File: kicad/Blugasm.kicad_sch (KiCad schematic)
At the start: 46 parts, among them J1 PWR, J2 OLED, J3 I2C, J4 SERVO1, J5 PJ-102AH, J6 SERVO2, J7 BATT, Q1 DMG3415U, Q2 Q_NMOS_DGS, SW1 PWR, SW2 PEC11R-4225F-50024, U1 MCP73831-2-OT, U2 MP3V5050GP, U3 MCP6001-OT, U4 AP2112K-3.3

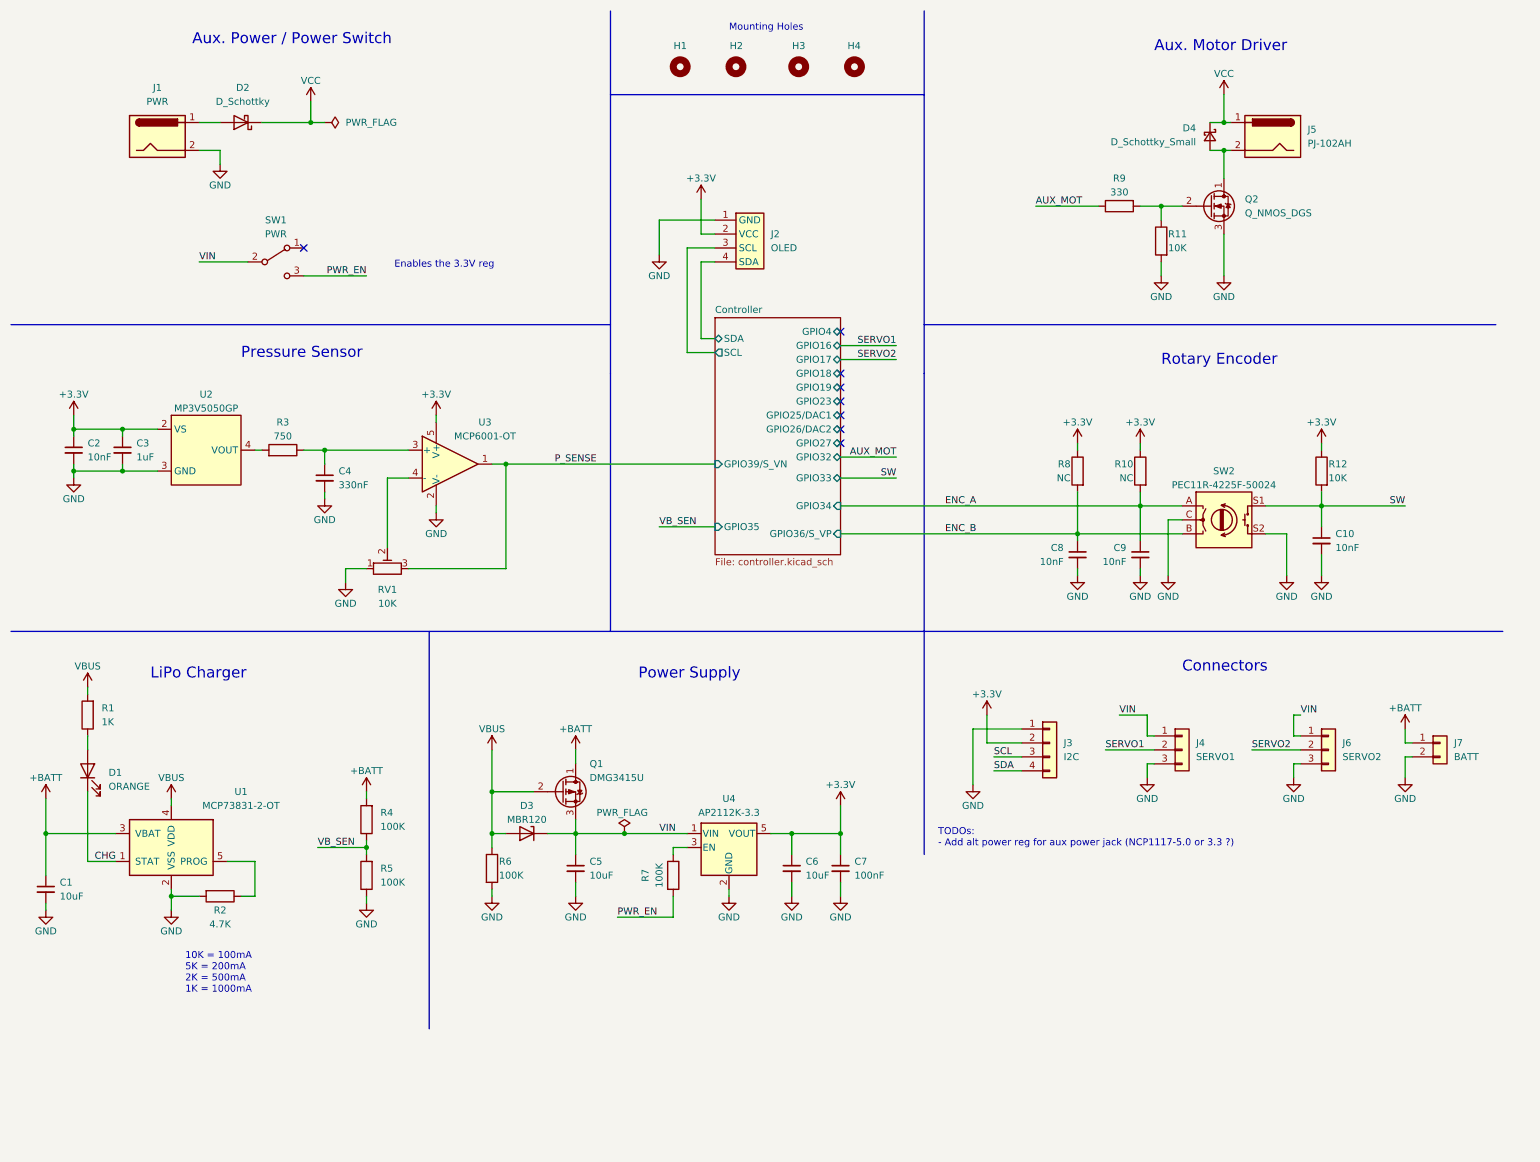
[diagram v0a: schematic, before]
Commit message: cleanup
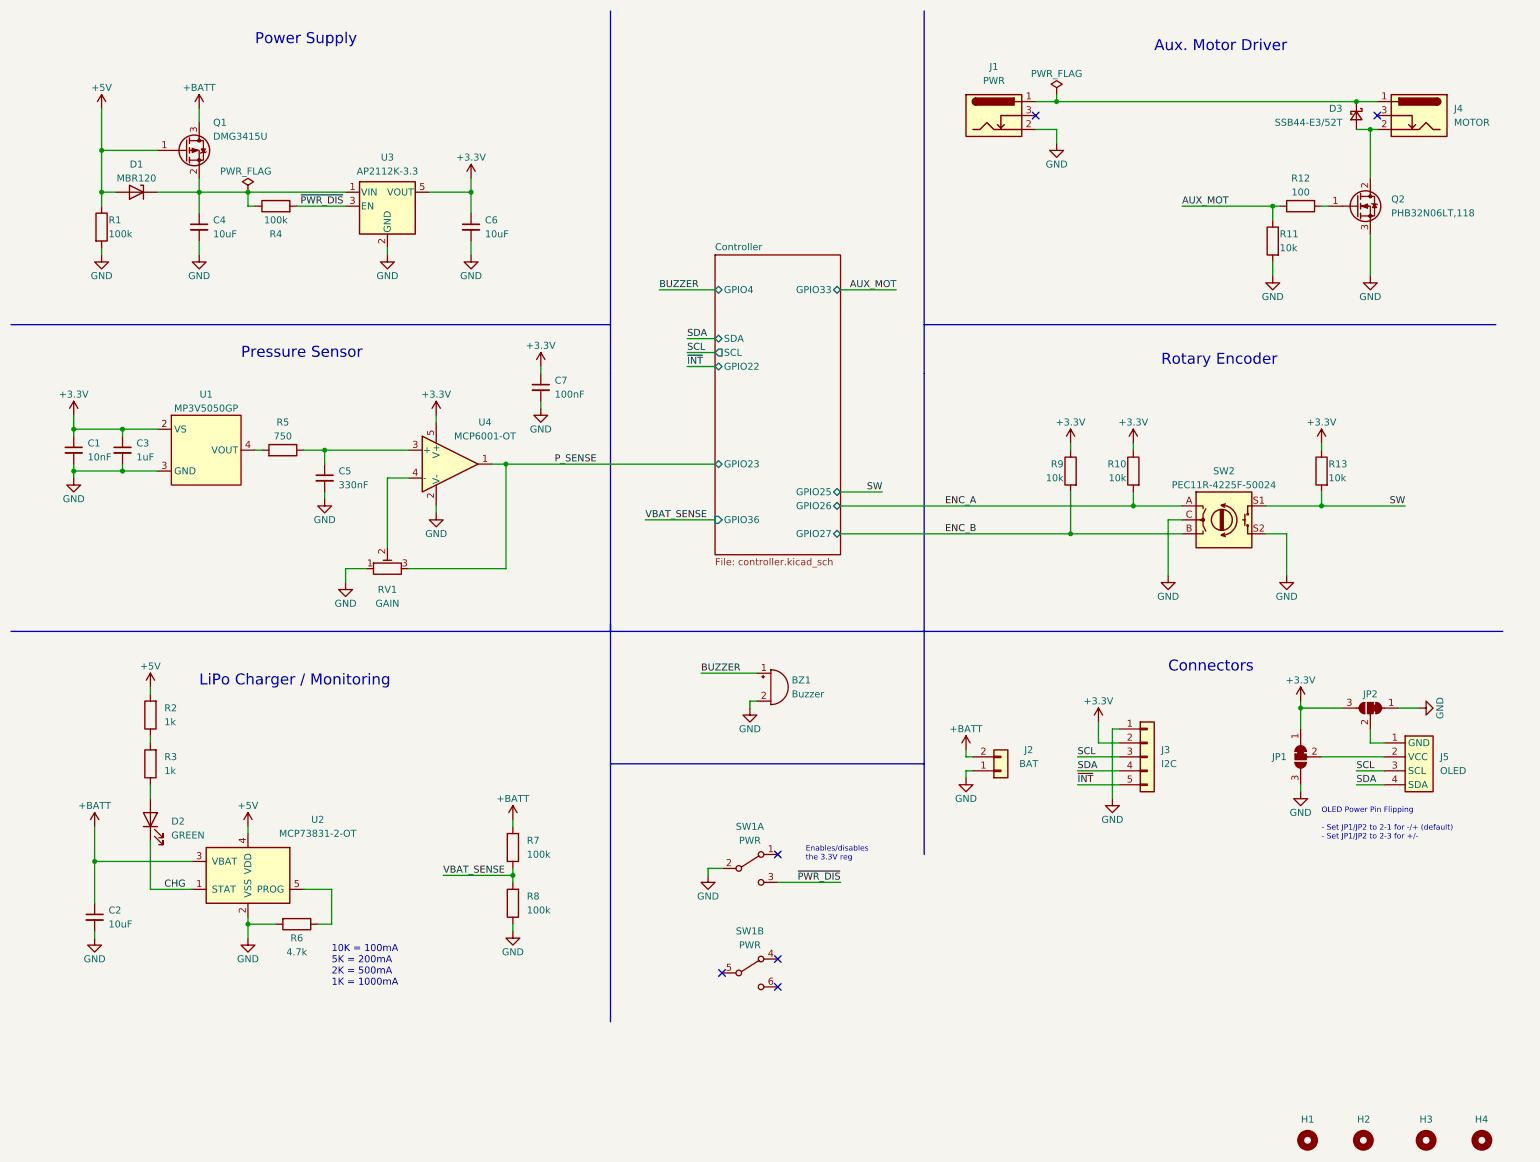
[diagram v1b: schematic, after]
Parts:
- removed C10, C8, C9: 10nF, Capacitor_SMD:C_0603_1608Metric, symbol Device:C_Small
- removed D2: D_Schottky, Diode_SMD:D_SOD-123, symbol Device:D_Schottky
- removed J4: SERVO1, Connector_PinHeader_2.54mm:PinHeader_1x03_P2.54mm_Vertical, symbol Connector_Generic:Conn_01x03
- removed J6: SERVO2, Connector_PinHeader_2.54mm:PinHeader_1x03_P2.54mm_Vertical, symbol Connector_Generic:Conn_01x03
- removed SW1: PWR, Button_Switch_THT:SW_E-Switch_EG2219_DPDT_Angled, symbol Switch:SW_SPDT
- added BZ1: Buzzer, Buzzer_Beeper:Buzzer_12x9.5RM7.6, symbol Device:Buzzer
- added JP1, JP2: SolderJumper_3_Bridged12, Jumper:SolderJumper-3_P1.3mm_Bridged12_Pad1.0x1.5mm_NumberLabels, symbol Jumper:SolderJumper_3_Bridged12
- added R2: 1k, Resistor_SMD:R_0603_1608Metric, symbol Device:R
- added SW1: PWR, Button_Switch_THT:SW_E-Switch_EG2219_DPDT_Angled, symbol Switch:SW_DPDT_x2
- C1: renamed from C2; MPN (none) -> CL10B103KB8NNNC
- C2: renamed from C1; MPN (none) -> CL10A106MA8NRNC
- C3: MPN (none) -> CL10B105KA8NFNC
- C4: renamed from C5; MPN (none) -> CL10A106MA8NRNC
- C5: renamed from C4; MPN (none) -> CL10B334KO8NNNC
- C6: MPN (none) -> CL10A106MA8NRNC
- C7: MPN (none) -> CL10B104KB8NNWC
- D1: renamed from D3; MPN (none) -> MBR120ESFT1G
- D2: renamed from D1; value ORANGE -> GREEN; MPN (none) -> 150060VS75000
- D3: renamed from D4; value D_Schottky_Small -> SSB44-E3/52T; MPN (none) -> SSB44-E3/52T
- J1: symbol Connector:Barrel_Jack -> Connector:Barrel_Jack_Switch; MPN (none) -> PJ-102AH
- J2: renamed from J7; value BATT -> BAT
- J3: footprint Connector_PinHeader_2.54mm:PinHeader_1x04_P2.54mm_Vertical -> Connector_PinHeader_2.54mm:PinHeader_1x05_P2.54mm_Horizontal; symbol Connector_Generic:Conn_01x04 -> Connector_Generic:Conn_01x05
- J4: renamed from J5; value PJ-102AH -> MOTOR; symbol Connector:Barrel_Jack -> Connector:Barrel_Jack_Switch; MPN (none) -> PJ-102AH
- Q1: symbol Device:Q_PMOS_DGS -> Device:Q_PMOS_GSD; MPN (none) -> DMG3415UQ-7
- Q2: value Q_NMOS_DGS -> PHB32N06LT,118; footprint Package_TO_SOT_SMD:SOT-223-3_TabPin2 -> Package_TO_SOT_SMD:TO-263-3_TabPin2; symbol Device:Q_NMOS_DGS -> Device:Q_NMOS_GDS; MPN (none) -> PHB32N06LT,118
- R1: renamed from R6; value 100K -> 100k; MPN (none) -> RC0603FR-07100KL
- R10: value NC -> 10k; MPN (none) -> RC0603FR-0710KL
- R11: value 10K -> 10k; MPN (none) -> RC0603FR-0710KL
- R12: renamed from R9; value 330 -> 100; MPN (none) -> RC0603FR-07100RL
- R13: renamed from R12; value 10K -> 10k; MPN (none) -> RC0603FR-0710KL
- R3: renamed from R1; value 1K -> 1k; MPN (none) -> RC0603FR-071KL
- R4: renamed from R7; value 100K -> 100k; MPN (none) -> RC0603FR-07100KL
- R5: renamed from R3; MPN (none) -> RC0603FR-07750RL
- R6: renamed from R2; value 4.7K -> 4.7k; MPN (none) -> RC0603FR-074K7L
- R7: renamed from R4; value 100K -> 100k; MPN (none) -> RC0603FR-07100KL
- R8: renamed from R5; value 100K -> 100k; MPN (none) -> RC0603FR-07100KL
- R9: renamed from R8; value NC -> 10k; MPN (none) -> RC0603FR-0710KL
- RV1: value 10K -> GAIN; footprint Resistor_SMD:R_0603_1608Metric -> SaawLib:ST-4EB; MPN (none) -> ST-4ETB103
- U1: renamed from U2; footprint (none) -> SaawLib:MP3V5050; MPN (none) -> MP3V5050GP
- U2: renamed from U1; MPN (none) -> MCP73831T-2ACI/OT
- U3: renamed from U4; MPN (none) -> AP2112K-3.3TRG1
- U4: renamed from U3; MPN (none) -> MCP6001RT-I/OT
- renumbered J2 to J5
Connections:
- net Controller/SCL is gone; now on net SCL: J5.3 (SCL)
- net Controller/SDA is gone; now on net SDA: J5.4 (SDA)
- net VCC is gone; now on an unnamed net: D3.1 (K), J4.1
- net +BATT: now also J2.2 (Pin_2), Q1.3 (D); no longer J2.1 (Pin_1), Q1.1 (D)
- net AUX_MOT: now also R11.1
- net GND: now also J2.1 (Pin_1), BZ1.2 (+), JP1.3 (B), JP2.1 (A), SW1.2 (B); no longer J2.2 (Pin_2), J5.1 (GND)
- net at D3.2 (A), J4.2: now also Q2.2 (D); no longer Q2.1 (D)
- net at R4.1: now also C4.1, D1.1 (K), Q1.2 (S), U3.1 (VIN); no longer U3.3 (EN)
- net +3V3 renamed +3.3V
- net +3.3V: now also JP1.1 (A), JP2.3 (B); no longer J5.2 (VCC)
- net PWR_EN renamed ~{PWR_DIS}
- net ~{PWR_DIS}: now also U3.3 (EN), SW1.3 (C)
- net VBUS renamed +5V
- net +5V: now also Q1.1 (G), R2.2; no longer Q1.2 (G), R3.2
- net VB_SEN renamed VBAT_SENSE
- removed net VIN: C4.1, D1.1 (K), Q1.3 (S), U3.1 (VIN)
- new net: J5.1 (GND), JP2.2 (C)
- new net: Q2.1 (G), R12.2
- new net: R2.1, R3.2
- new net: J5.2 (VCC), JP1.2 (C)
- new net BUZZER: BZ1.1 (-)
- new net ~{INT}: J3.5 (Pin_5)
- no-connect marks 8 -> 6
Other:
- sheet Controller ports: added GPIO22, GPIO25, GPIO26, GPIO36; removed GPIO16, GPIO17, GPIO18, GPIO19, GPIO25/DAC1, GPIO26/DAC2, GPIO32, GPIO34, GPIO35, GPIO36/S_VP, GPIO39/S_VN
- note added: "Enables/disables the 3.3V reg"
- note added: "LiPo Charger / Monitoring"
- note added: "OLED Power Pin Flipping - Set JP1/JP2 to 2-1 for -/+ (default) - Set JP1/JP2 to 2-3 for +/-"
- note removed: "Aux. Power / Power Switch"
- note removed: "Enables the 3.3V reg"
- note removed: "LiPo Charger"
- note removed: "Mounting Holes"
- note removed: "TODOs: - Add alt power reg for aux power jack (NCP1117-5.0 or 3.3 ?)"
- company: (none) -> saawsm
- moved on the sheet: C2, C4, C6, D1, D2, D3, H1, H2, H3, H4, J2, J5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
